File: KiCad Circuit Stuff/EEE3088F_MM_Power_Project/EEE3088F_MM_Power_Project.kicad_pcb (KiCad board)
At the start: 2 copper layers, 77.3 x 58.5 mm, 88 parts, among them J1 Conn_01x02, J2 Conn_02x16_Odd_Even, U1 MT3608, U10 DRV8833PWP, U11 SS-12D06-G050, U12 AP22814AW5-7, U14 AP22814AW5-7, U2 INA219AIDCNR, U3 AMS1117-3.3, U4 TPS5430DDAR, U5 TP4056, U6 TS5A3159DCKR, U7 TYPE-C_16P_QTGM027, U8 DRV8833PWP, U9 HUSB237-AA001-DN06R

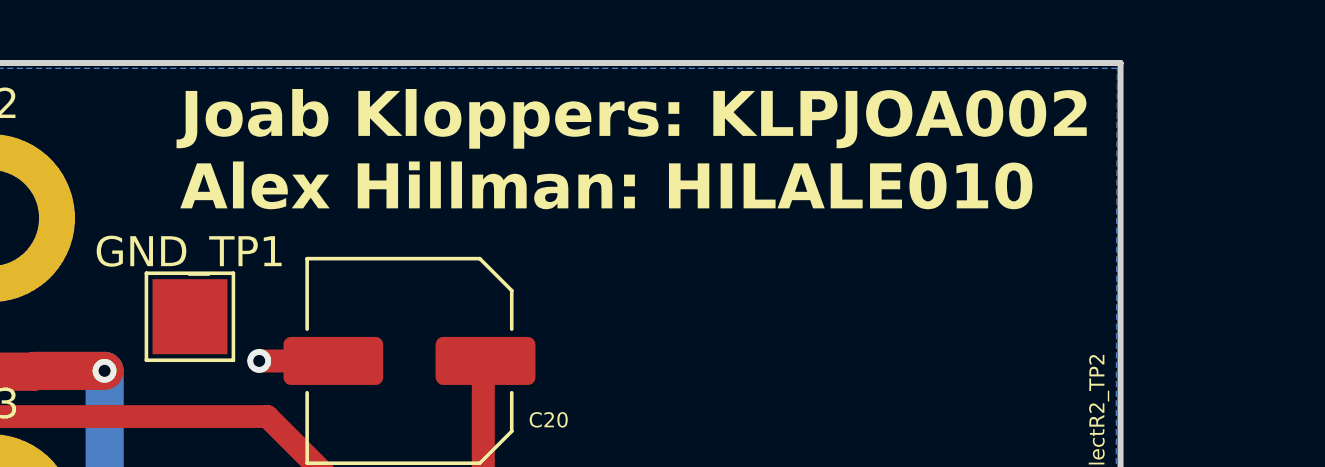
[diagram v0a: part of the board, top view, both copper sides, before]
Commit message: added stuff
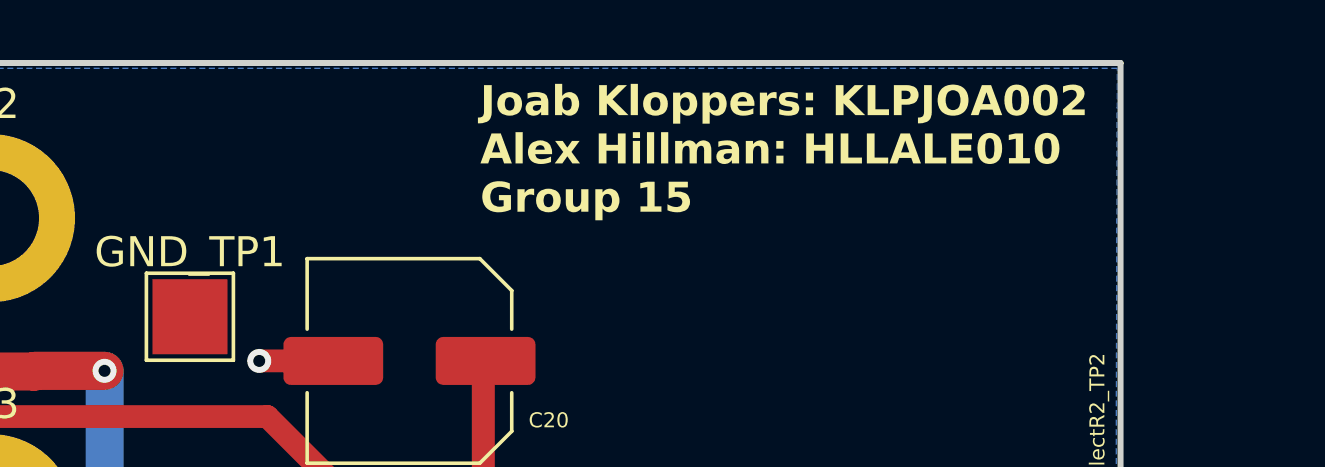
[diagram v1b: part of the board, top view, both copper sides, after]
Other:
- board text added: "Joab Kloppers: KLPJOA002 Alex Hillman: HLLALE010 Group 15"
- board text removed: "Joab Kloppers: KLPJOA002 Alex Hillman: HILALE010"
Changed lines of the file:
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@@
     (property "ki_description" "Generic connector, single row, 01x02, script generated (kicad-library-utils/schlib/autogen/connector/)")
     (property "ki_keywords" "connector")
-    (attr through_hole)
+    (attr through_hole exclude_from_bom)
     (fp_text reference "J1" (at 1 -2.9 90) (layer "F.SilkS")
         (effects (font (size 1 1) (thickness 0.15)))
@@
     (property "ki_description" "Generic connector, double row, 02x16, odd/even pin numbering scheme (row 1 odd numbers, row 2 even numbers), script generated (kicad-library-utils/schlib/autogen/connector/)")
     (property "ki_keywords" "connector")
-    (attr through_hole)
+    (attr through_hole exclude_from_bom)
     (fp_text reference "J2" (at 1.27 -2.33 90) (layer "F.SilkS")
         (effects (font (size 1 1) (thickness 0.15)))
@@
   (gr_rect (start 100 94.4882) (end 177.3 152.95)
     (stroke (width 0.2) (type default)) (fill none) (layer "Edge.Cuts"))
-  (gr_text "Joab Kloppers: KLPJOA002\nAlex Hillman: HILALE010\n" (at 145.9484 99.5172) (layer "F.SilkS")
-    (effects (font (size 1.5 1.5) (thickness 0.3) bold) (justify left bottom))
+  (gr_text "Joab Kloppers: KLPJOA002\nAlex Hillman: HLLALE010\nGroup 15\n" (at 155.956 99.568) (layer "F.SilkS")
+    (effects (font (size 1 1) (thickness 0.2) bold) (justify left bottom))
   )
   (segment (start 137.499863 116.76147) (end 137.46713 116.76147) (width 0.76) (layer "F.Cu") (net 1))
